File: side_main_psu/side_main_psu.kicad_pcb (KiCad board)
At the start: 2 copper layers, 94 x 53.5 mm, 35 parts, among them J101 Conn_01x02, J103 Conn_01x02, Q301 IXTP28P065T, Q302 TK4R3E06PL, U301 LT8710

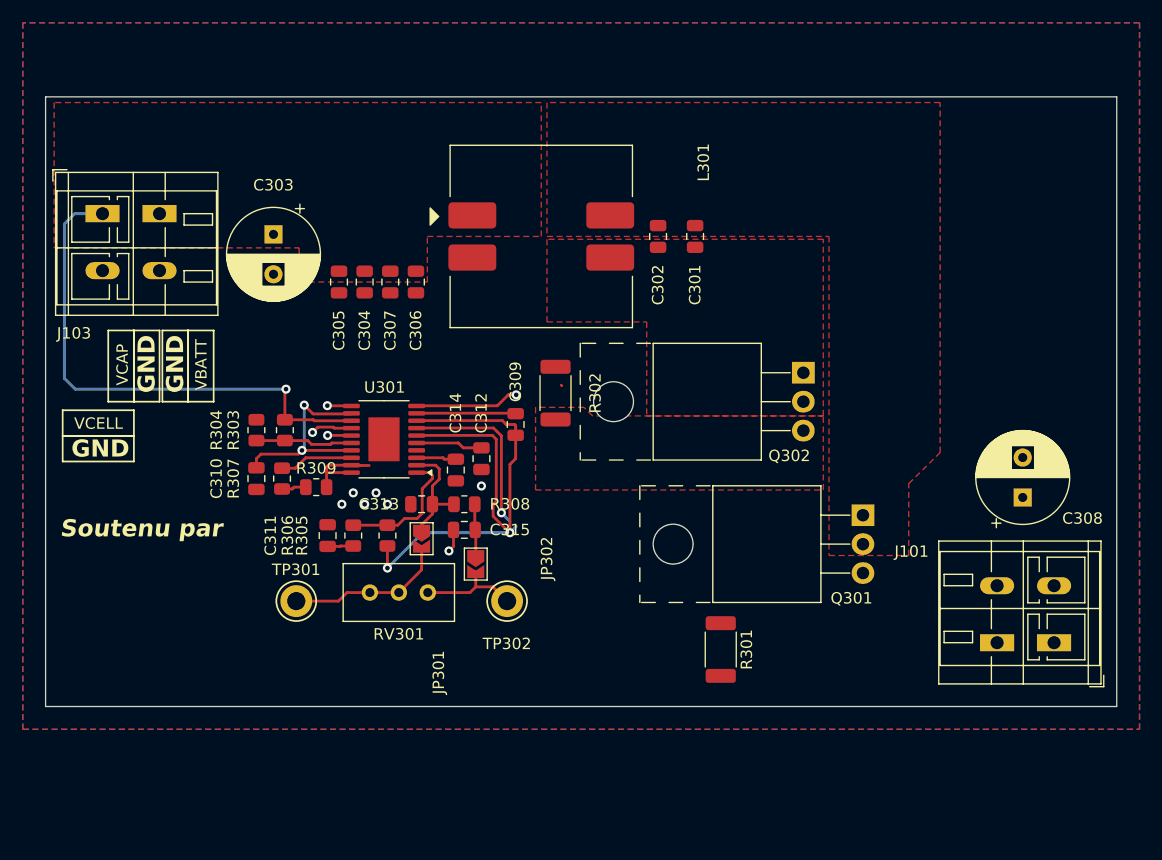
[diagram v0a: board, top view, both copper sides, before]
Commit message: Start soft with vscode and STM32 extension
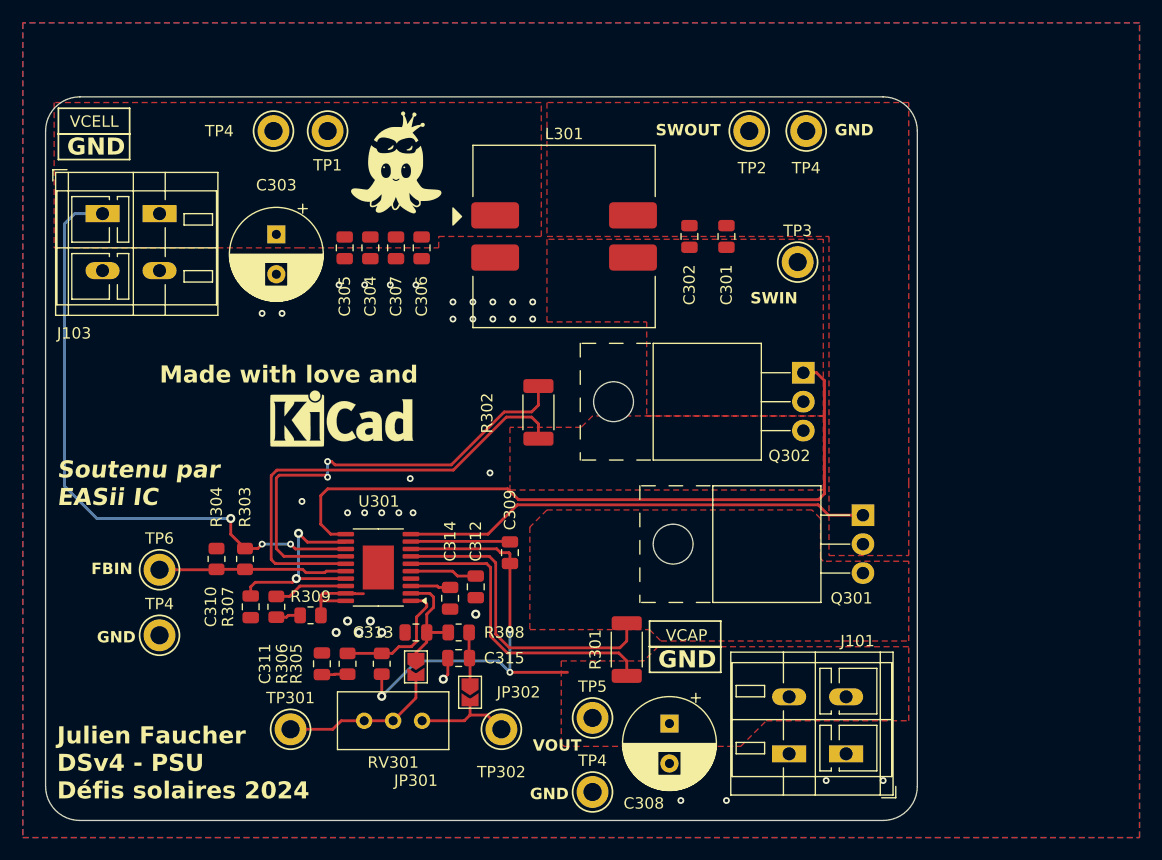
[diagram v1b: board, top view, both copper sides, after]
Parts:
- added G***: LOGO, LOGO, F.Cu at (130.8, 51.2)
- added REF**: KiCad-Logo_5mm_SilkScreen, Symbol:KiCad-Logo_5mm_SilkScreen, F.Cu at (126.0, 74.2)
- added TP1: TP_VIN, TestPoint:TestPoint_Keystone_5010-5014_Multipurpose, F.Cu at (124.8, 48.5)
- added TP2: TP_SWOUT, TestPoint:TestPoint_Keystone_5010-5014_Multipurpose, F.Cu at (161.8, 48.5)
- added TP3: TP_SWIN, TestPoint:TestPoint_Keystone_5010-5014_Multipurpose, F.Cu at (166.0, 60.0)
- added TP4: TP_GND, TestPoint:TestPoint_Keystone_5010-5014_Multipurpose, F.Cu at (110.0, 92.8)
- added TP4: TP_GND, TestPoint:TestPoint_Keystone_5010-5014_Multipurpose, F.Cu at (166.8, 48.5)
- added TP4: TP_GND, TestPoint:TestPoint_Keystone_5010-5014_Multipurpose, F.Cu at (120.0, 48.5)
- added TP4: TP_GND, TestPoint:TestPoint_Keystone_5010-5014_Multipurpose, F.Cu at (148.0, 106.5)
- added TP5: TP_VOUT, TestPoint:TestPoint_Keystone_5010-5014_Multipurpose, F.Cu at (148.0, 100.0)
- added TP6: TP_FBIN, TestPoint:TestPoint_Keystone_5010-5014_Multipurpose, F.Cu at (110.0, 87.0)
- moved C308 36.8 mm to (154.8, 100.5), turned to -90 degrees
- moved J101 20.7 mm to (165.2, 103.2)
- moved R303 11.8 mm to (117.5, 86.0)
- moved R304 11.8 mm to (115.0, 86.0)
- moved C309 11.3 mm to (140.8, 85.5)
- moved C310 11.3 mm to (118.0, 90.2)
- moved C311 11.3 mm to (124.2, 95.2)
- moved C312 11.3 mm to (137.8, 88.5)
- moved C313 11.3 mm to (132.5, 92.5)
- moved C314 11.3 mm to (135.5, 89.5)
- moved C315 11.3 mm to (136.2, 94.8)
- moved JP301 11.3 mm to (132.5, 95.5)
- moved JP302 11.3 mm to (137.2, 97.8)
- moved R305 11.3 mm to (129.5, 95.2)
- moved R306 11.3 mm to (126.5, 95.2)
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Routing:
- net Net-(Q302-G): track 2.10 -> 62.2 mm, vias 1 -> 0
- net /PSU Core/SWIN_CSP: track 2.07 -> 41.2 mm, vias 1 -> 0
- net PGND: track 13.5 -> 50.9 mm, vias 8 -> 37
- net Net-(Q301-G): track 9.12 -> 41.1 mm, vias 1 -> 0
- net /PSU Core/V_{OUT}: track 49.3 -> 66.5 mm, vias 2 -> 3
- net /PSU Core/SWOUT_ISP: track 15.5 -> 27.7 mm, vias 1 -> 0
- net /PSU Core/V_{IN}: track 45.7 -> 54.8 mm, vias 1 -> 3
- net Net-(U301-EN/FBIN): track 8.53 -> 16.5 mm
- added copper zone on F.Cu, net /PSU Core/SWOUT_ISP
- added copper zone on F.Cu, net /PSU Core/V_{OUT}
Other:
- board size 94 x 53.5 mm -> 76.5 x 63.5 mm
- board text added: "FBIN"
- board text added: "Julien Faucher DSv4 - PSU Défis solaires 2024"
- board text added: "Made with love and"
- board text added: "Main PSU DSv4 for défis solaires 2024 Octocar - Julien FAUCHER Input 14 SunPower solar cells in series. Output capacitors, 18V"
- board text added: "SWIN"
- board text added: "SWOUT"
- board text added: "Soutenu par EASii IC"
- board text added: "VOUT"
- board text removed: "Carte principale DSv4 pour défis solaires 2024 Octocar - Julien FAUCHER Entrée 14 Cellules solaires. Sortie condensateurs, 18V Sortie Li-Ion 3S1P 11.4V"
- board text removed: "Soutenu par"
- board text removed: "VBATT"
